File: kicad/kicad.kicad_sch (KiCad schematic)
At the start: 2 parts, among them U1 AS6C1616, U2 AS6C1616

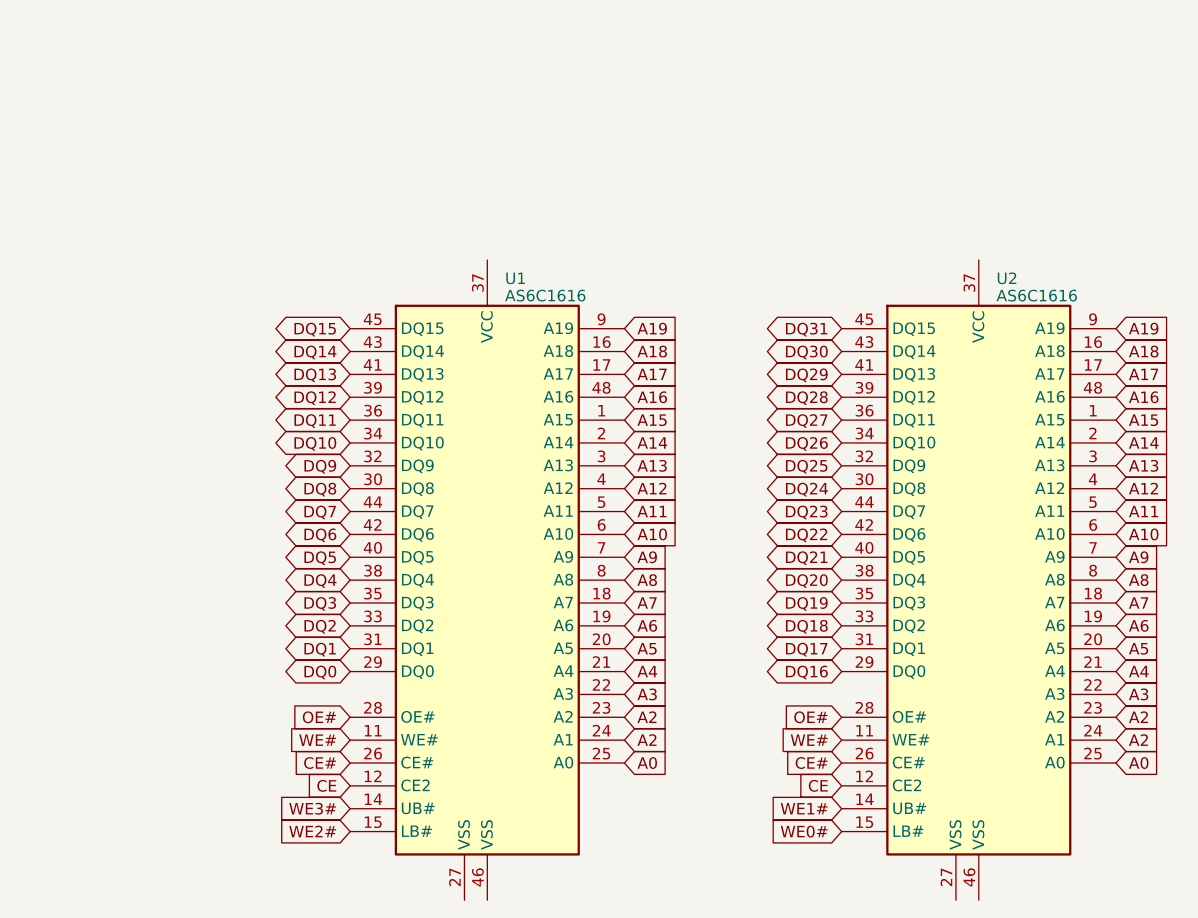
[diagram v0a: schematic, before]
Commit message: Add concat
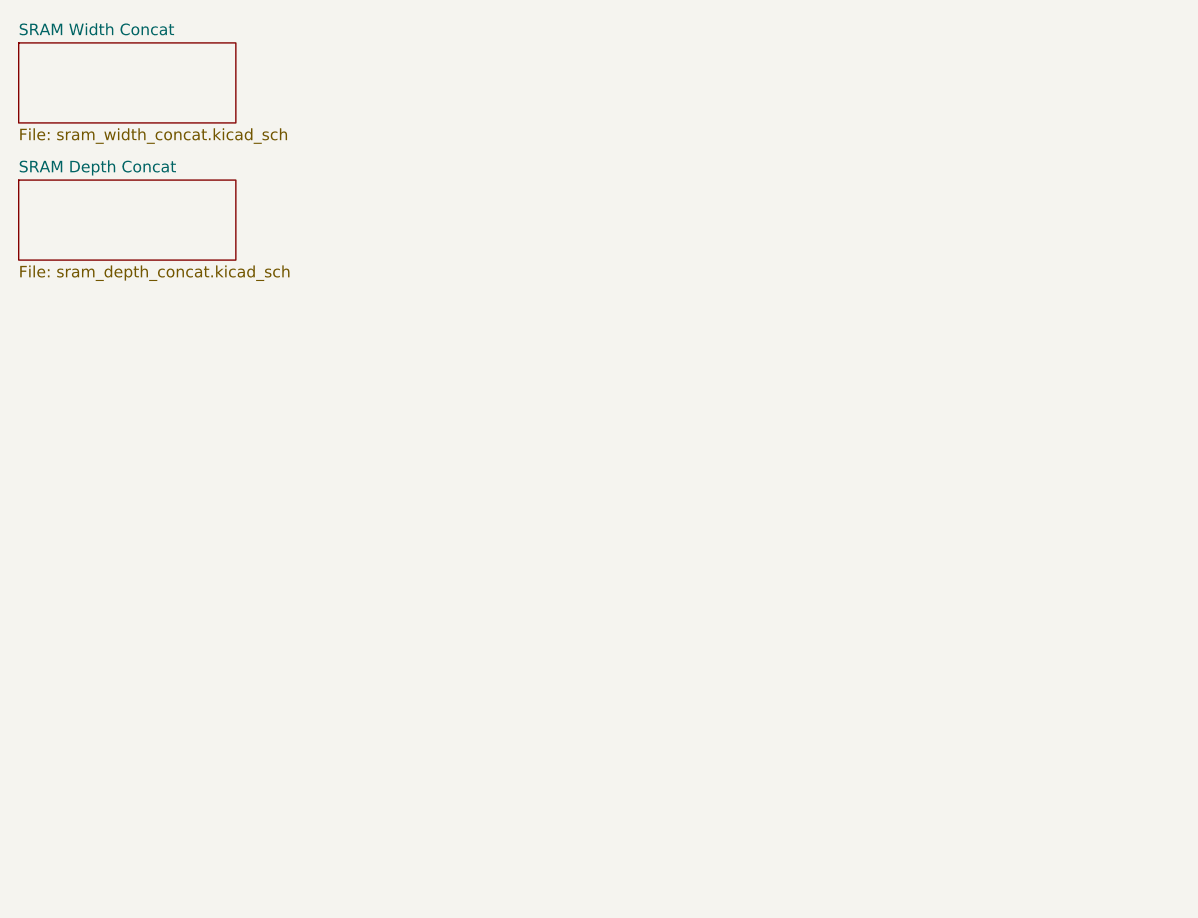
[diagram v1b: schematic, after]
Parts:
- removed U1, U2: AS6C1616, Package_SO:TSOP-I-48_18.4x12mm_P0.5mm, symbol Memory_RAM:AS6C1616
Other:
- added sheet SRAM Depth Concat (sram_depth_concat.kicad_sch)
- added sheet SRAM Width Concat (sram_width_concat.kicad_sch)
